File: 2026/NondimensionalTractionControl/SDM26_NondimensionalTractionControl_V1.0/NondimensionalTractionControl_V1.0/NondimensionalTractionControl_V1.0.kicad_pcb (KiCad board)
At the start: 4 copper layers, 50 x 50 mm, 52 parts, among them IC1 STM32H743VIT6, IC2 74LVC1G17SE-7, IC3 TLP175A_TPL,E, IC4 SN65HVD230QDR, IC5 TPS259250DRCR, IC6 MIC37100-3.3WS, IC7 TPS2116DRLR, J1 104031-0811, J2 Conn_ARM_SWD_TagConnect_TC203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, J3 105017-0001, J4 SM04B-ULHK-1TA1-ETB_HF_, J5 SM04B-ULHK-1TA1-ETB_HF_, J6 SM04B-ULHK-1TA1-ETB_HF_, U1 USBLC6-2SC6, Y1 ABM3B-8.000MHZ-10-1-U-T

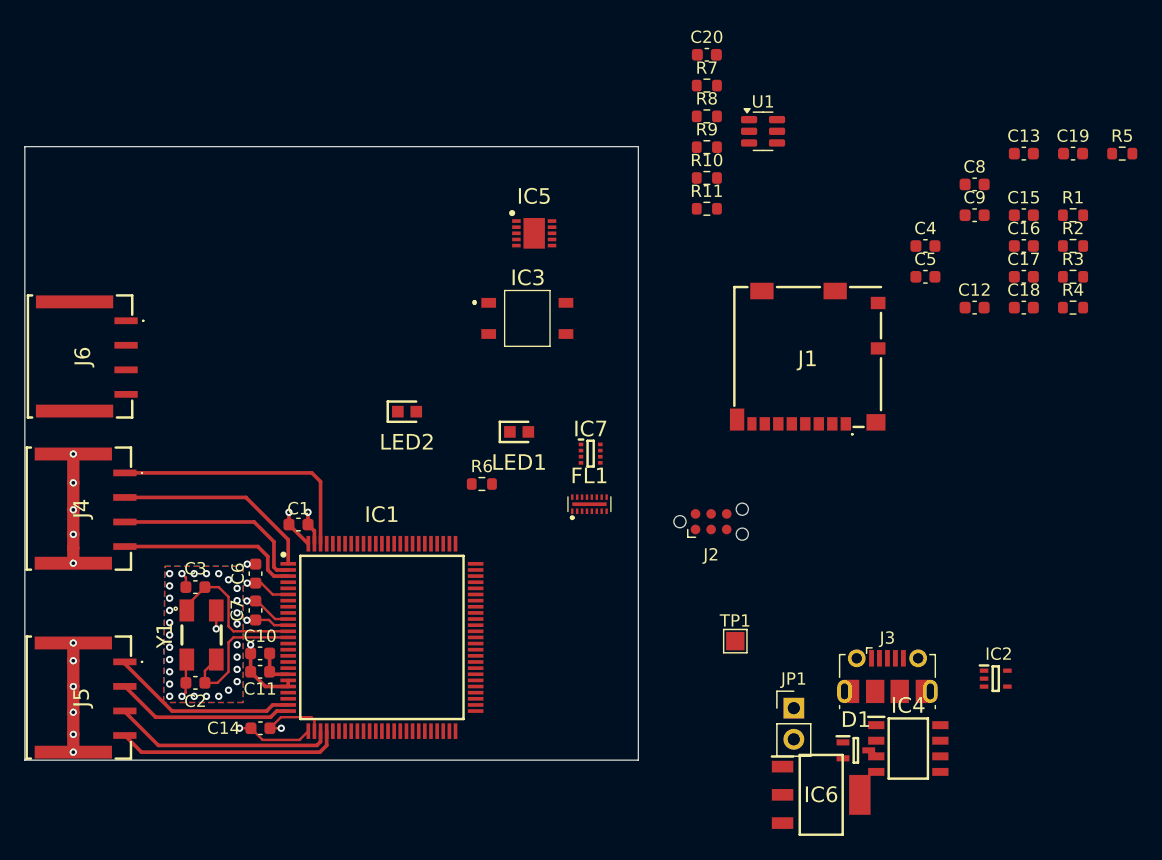
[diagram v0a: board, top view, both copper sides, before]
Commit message: NDTC PCB mostly done
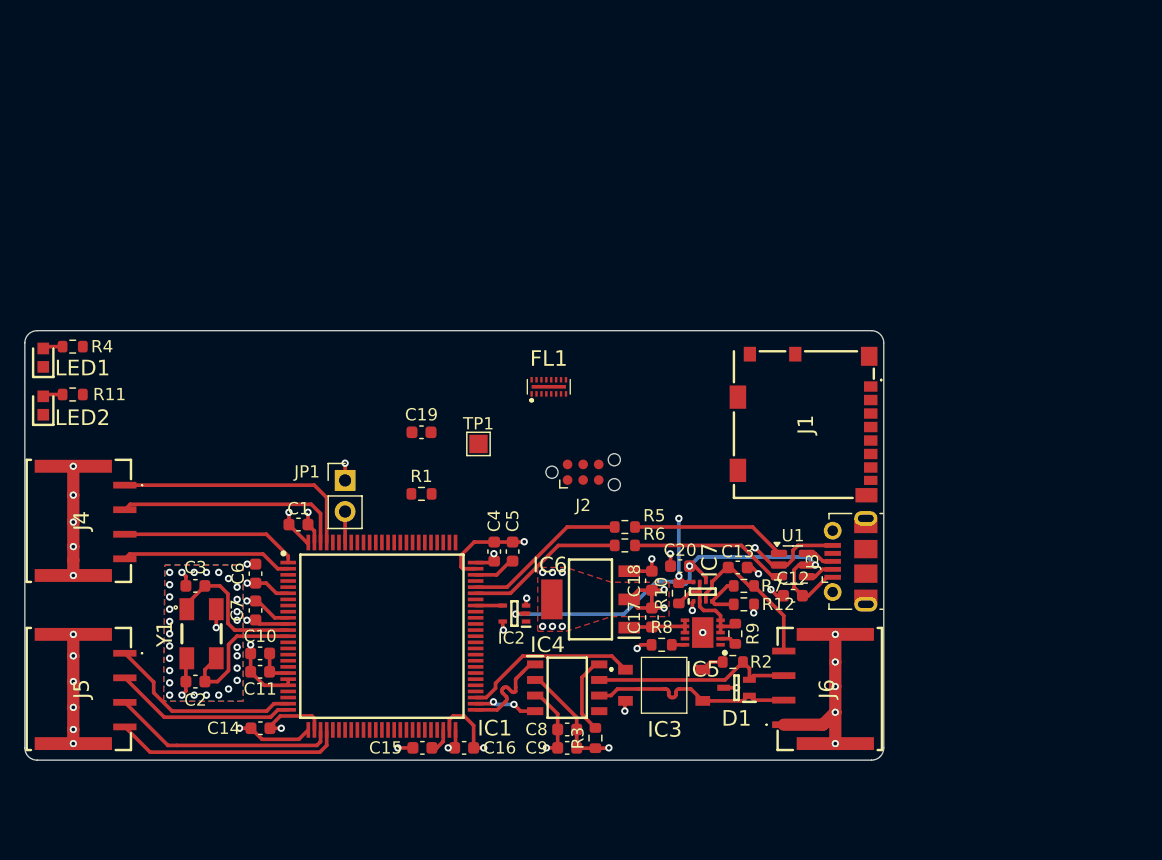
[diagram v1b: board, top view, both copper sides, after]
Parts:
- added R12: 10k, Resistor_SMD:R_0603_1608Metric, F.Cu at (158.6, 137.3)
- J3: value 105017-0001 -> USB_B_Micro
- moved R4 81.6 mm to (103.9, 116.3), turned to 180 degrees
- moved J6 66.8 mm to (165.6, 144.2), turned to -90 degrees
- moved C15 65.5 mm to (132.4, 149.0), turned to 180 degrees
- moved C16 61.3 mm to (135.8, 149.0), turned to 180 degrees
- moved C19 57.8 mm to (132.3, 123.3)
- moved R1 57.8 mm to (132.3, 128.3)
- moved C8 55.5 mm to (144.2, 147.5)
- moved C9 54.7 mm to (144.2, 149.0)
- moved R3 54.1 mm to (146.5, 148.2), turned to 90 degrees
- moved R11 53.9 mm to (103.9, 120.2), turned to 180 degrees
- moved R5 50.7 mm to (148.9, 131.0), turned to 180 degrees
- moved R2 43.8 mm to (157.7, 142.0)
- moved R8 43.2 mm to (151.9, 140.6)
- moved C4 43.1 mm to (138.2, 133.0), turned to -90 degrees
- moved C20 41.7 mm to (153.4, 134.2), turned to 180 degrees
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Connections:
- IC1 pad 1: WheelSpeed_2 -> WheelSpeed_3
- IC1 pad 2: WheelSpeed_3 -> WheelSpeed_4
- IC1 pad 3: WheelSpeed_4 -> unconnected-(IC1-PE4-Pad3)
- IC1 pad 51: Net-(IC1-PB12) -> /FDCAN2_RX
- IC1 pad 52: unconnected-(IC1-PB13-Pad52) -> /FDCAN2_TX
- IC1 pad 53: unconnected-(IC1-PB14-Pad53) -> /CAN_TERM
- IC1 pad 54: unconnected-(IC1-PB15-Pad54) -> /USER_LED
- IC1 pad 95: /FDCAN1_RX -> unconnected-(IC1-PB8-Pad95)
- IC1 pad 96: /FDCAN1_TX -> unconnected-(IC1-PB9-Pad96)
- IC1 pad 97: /CAN_TERM -> WheelSpeed_1
- IC1 pad 98: WheelSpeed_1 -> WheelSpeed_2
- IC4 pad 1: /FDCAN1_RX -> /FDCAN2_RX
- IC4 pad 4: /FDCAN1_TX -> /FDCAN2_TX
- IC7 pad 4: GND -> Net-(IC7-PR1)
- J6 pad 1: VCC -> GND
- J6 pad 2: /CAN_HI -> /CAN_LOW
- J6 pad 3: /CAN_LOW -> /CAN_HI
- J6 pad 4: GND -> VCC
- R4 pad 1: Net-(IC1-PB12) -> /USER_LED
- R7 pad 2: GND -> Net-(IC7-PR1)
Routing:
- net GND: track 37.8 -> 100.4 mm, vias 45 -> 73
- net VBUS: track 0.00 -> 37.8 mm, vias 0 -> 3
- net /CAN_HI: track 0.00 -> 16.9 mm
- net /CAN_LOW: track 0.00 -> 16.9 mm
- net +3.3V: track 22.3 -> 37.4 mm, vias 5 -> 11
- net /CAN_TERM: track 0.00 -> 14.3 mm
- net /USB_OTG_DP: track 0.00 -> 13.4 mm
- net /USB_OTG_DM: track 0.00 -> 13.0 mm
- net VCC: track 0.00 -> 12.8 mm
- net Net-(R6-Pad2): track 0.00 -> 12.8 mm
- net Net-(R5-Pad1): track 0.00 -> 12.6 mm
- net +5V: track 0.00 -> 8.76 mm
- net /FDCAN2_RX: track 0.00 -> 8.34 mm
- net Net-(IC4-Rs): track 0.00 -> 6.58 mm
- net Net-(IC7-ST): track 0.00 -> 6.41 mm, vias 0 -> 2
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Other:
- board size 50 x 50 mm -> 70 x 35 mm
